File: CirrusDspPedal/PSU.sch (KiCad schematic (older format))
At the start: 9 parts, among them J4 Barrel_Jack_Switch, J7 Conn_01x01, U4 LD1117S50TR_SOT223, U5 MCP1703A-1202_SOT223

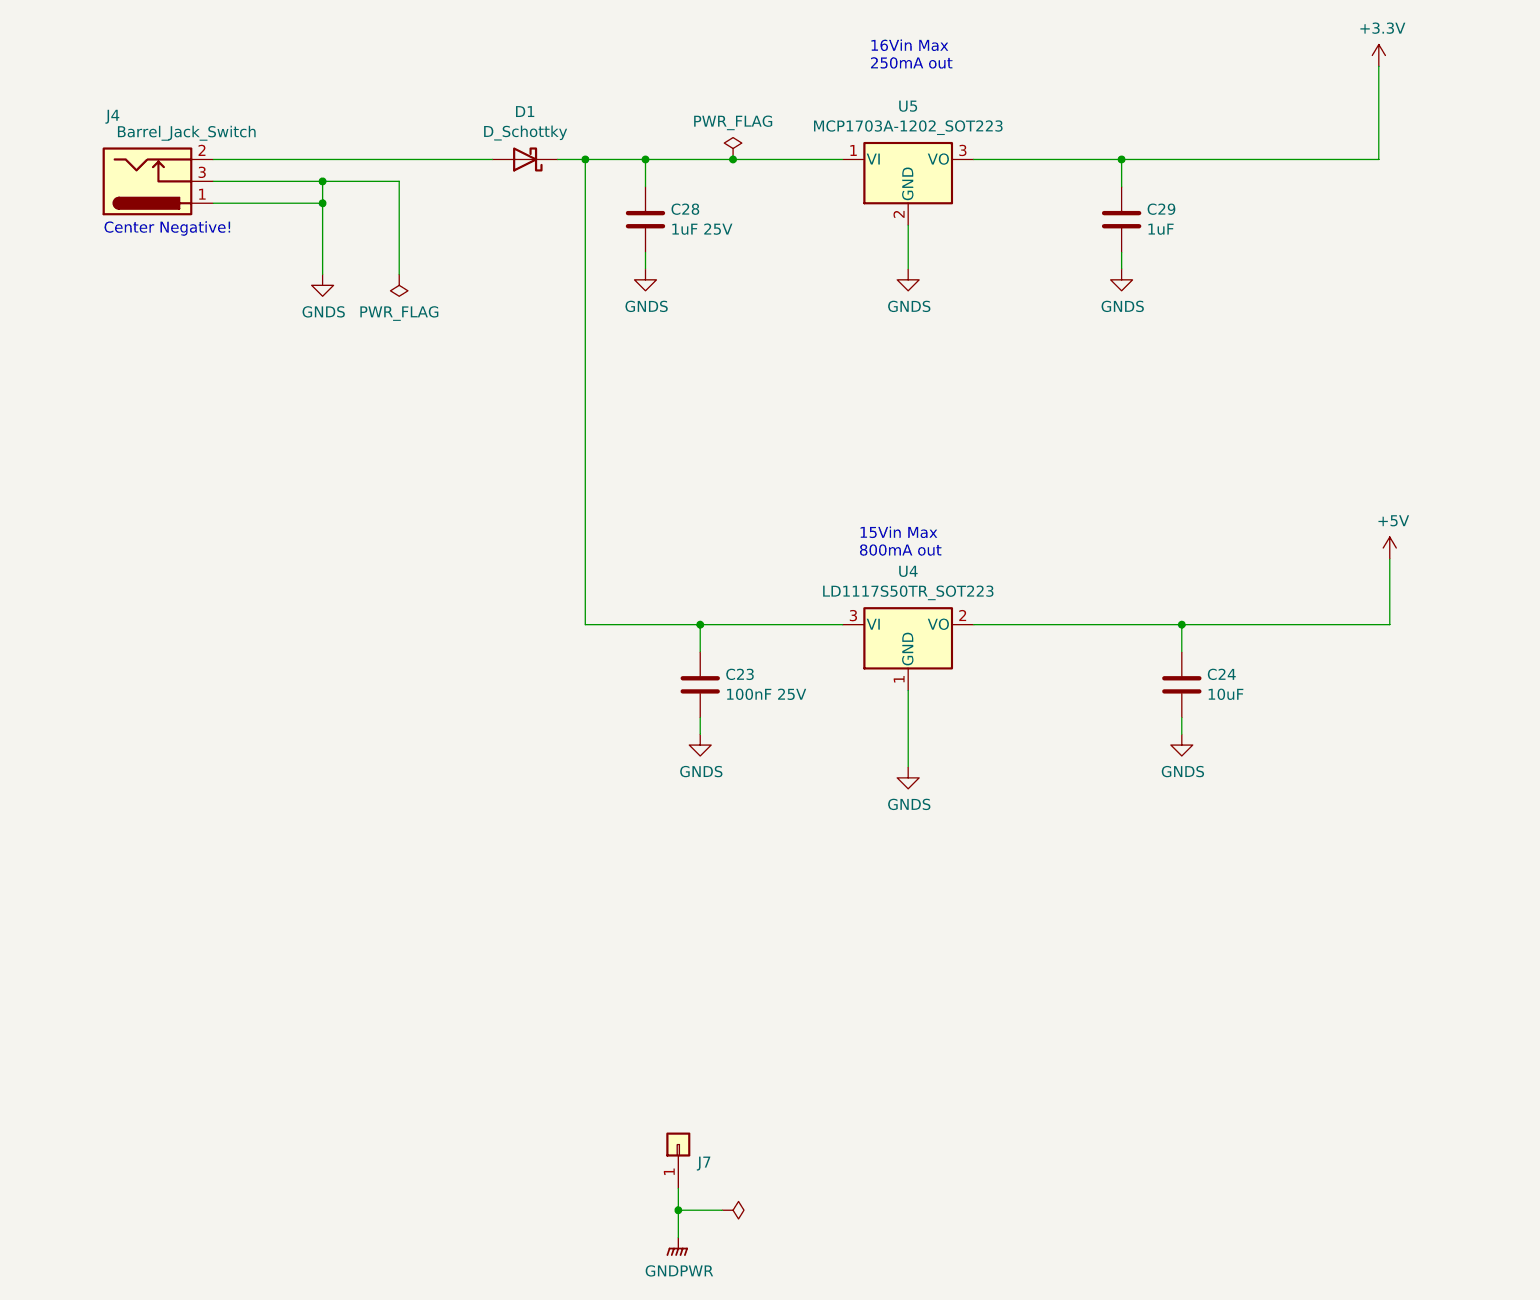
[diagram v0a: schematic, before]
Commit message: final revb layout
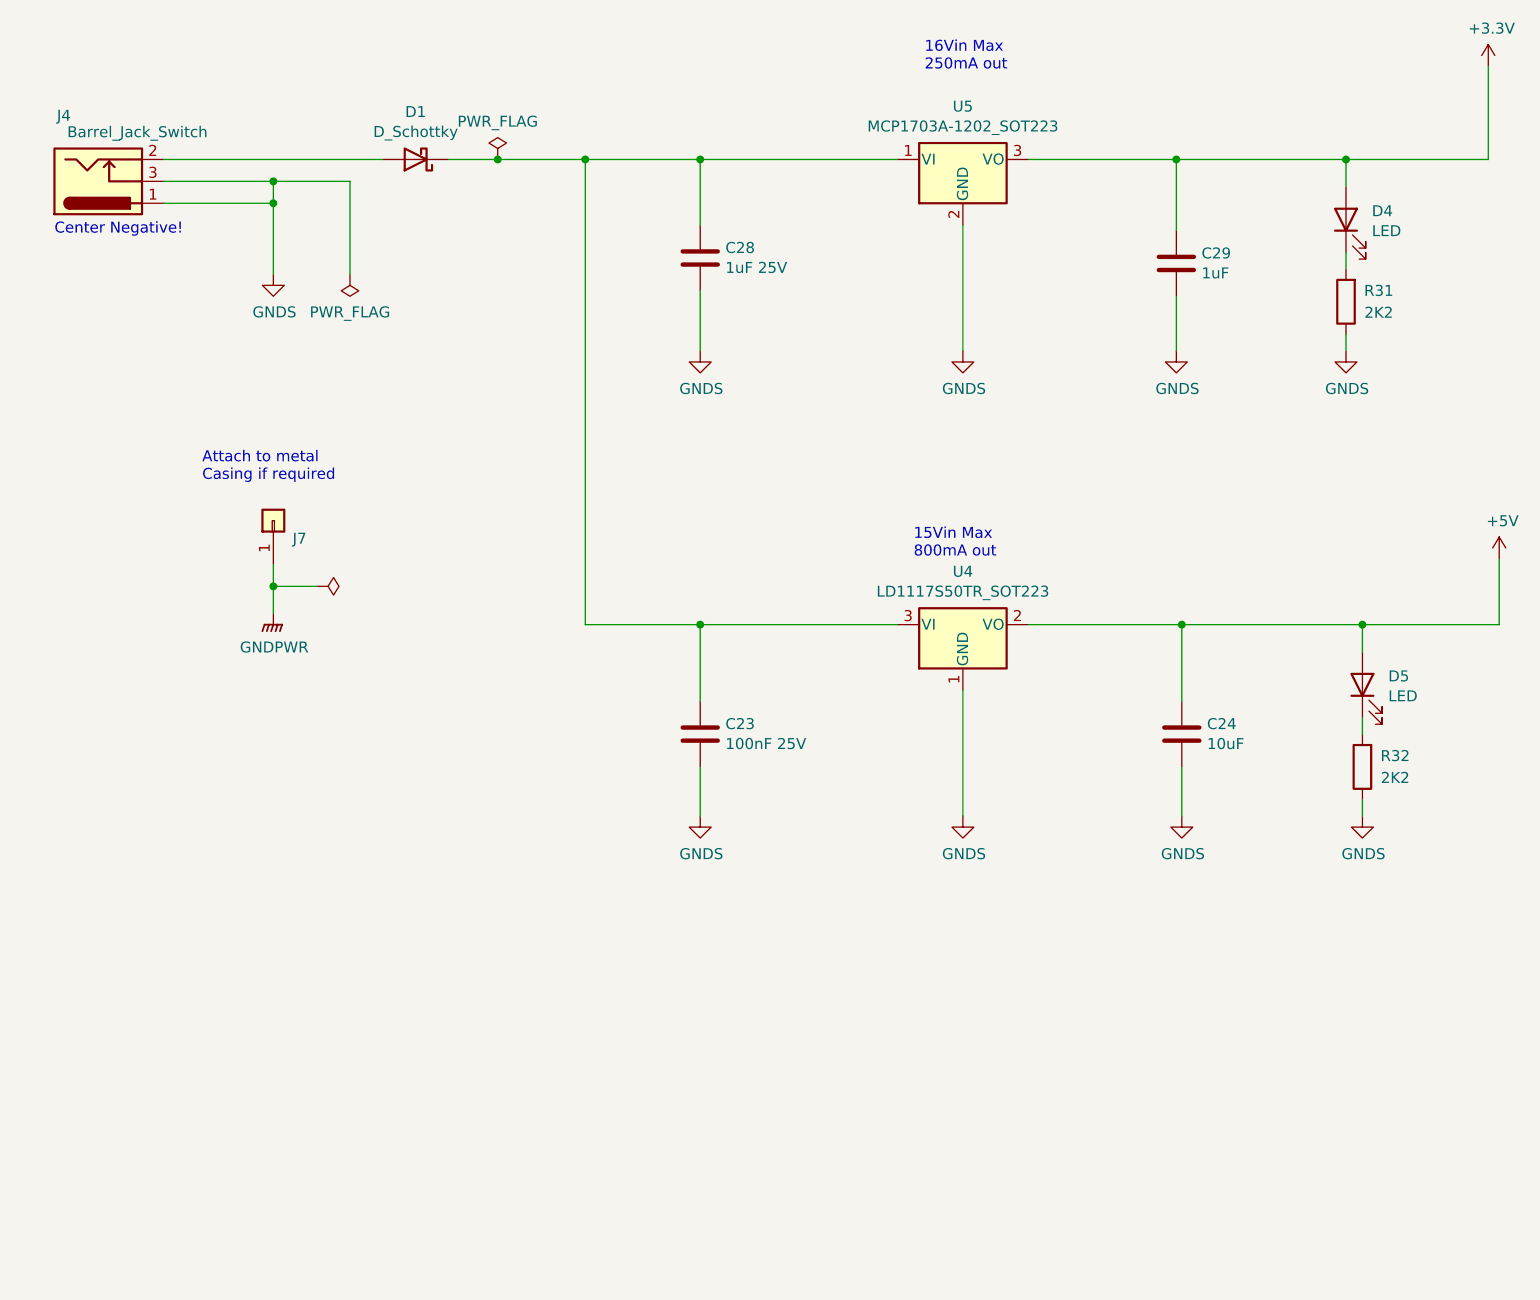
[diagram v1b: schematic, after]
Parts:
- added D4, D5: LED, LED_SMD:LED_0805_2012Metric_Pad1.15x1.40mm_HandSolder, symbol Device:LED
- added R31, R32: 2K2, Resistor_SMD:R_0805_2012Metric_Pad1.20x1.40mm_HandSolder, symbol Device:R
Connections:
- net +3V3: now also D4.2 (A)
- net +5V: now also D5.2 (A)
- net GNDS: now also R31.1, R32.1
- new net: D4.1 (K), R31.2
- new net: D5.1 (K), R32.2
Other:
- note added: "Attach to metal\nCasing if required"
- moved on the sheet: C23, C24, C28, C29, D1, J4, J7, U4, U5
